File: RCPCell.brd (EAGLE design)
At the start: 99.8 x 80 mm, 23 parts, among them IC1 SIM900, Q1 BSS84, Q2 BSS84, U1 PESDXS4UD

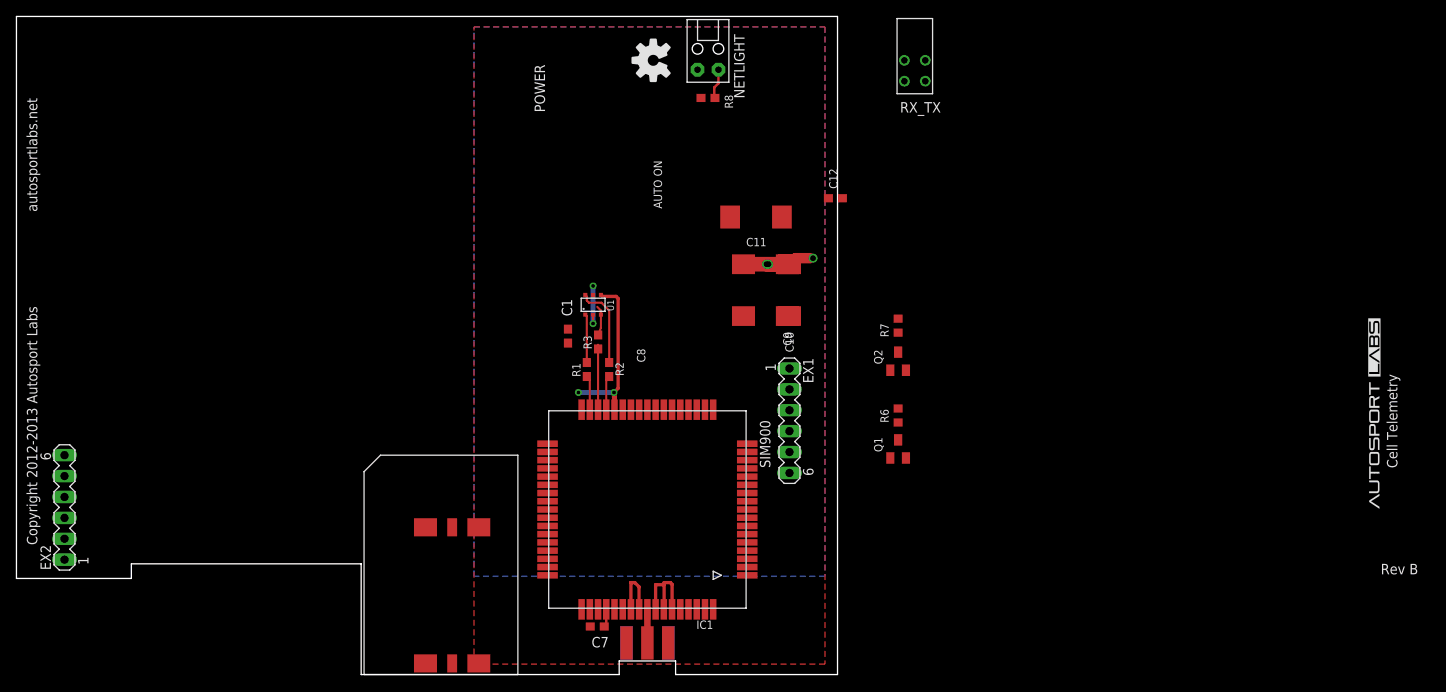
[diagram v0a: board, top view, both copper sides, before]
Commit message: WIP for MK2 version of cell module
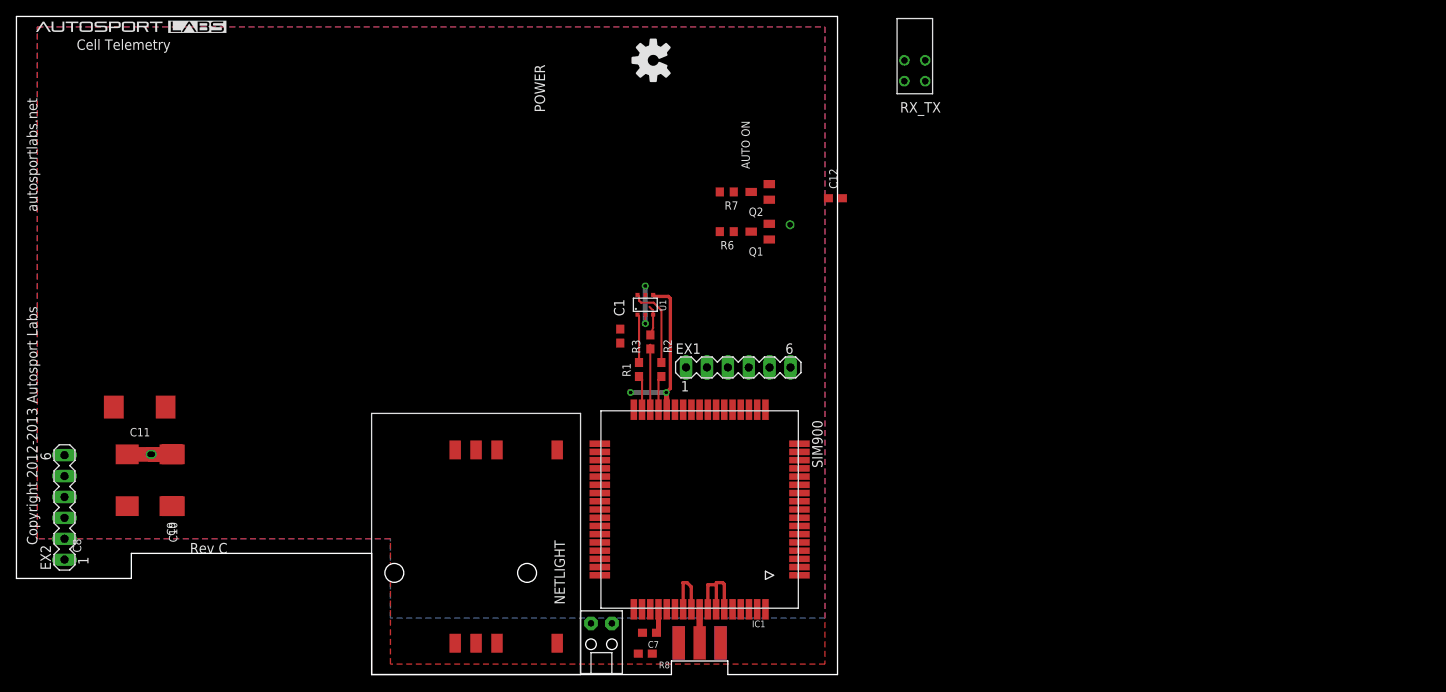
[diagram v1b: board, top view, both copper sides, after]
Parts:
- U$1: value MOLEX_0470230001 -> MOLEX_04702300012; device simcard:MOLEX_0470230001 -> simcard:MOLEX_91228-3001
- moved C10 78.4 mm to (19.1, 23.6)
- moved C9 78.4 mm to (18.8, 23.6)
- moved C11 78.4 mm to (15.0, 32.5)
- moved C8 78.4 mm to (13.5, 23.6)
- moved NETLIGHT 71.8 mm to (71.1, 4.57), turned to 0 degrees
- moved R8 68.0 mm to (76.5, 2.54)
- moved Q1 31.3 mm to (90.4, 53.8), turned to 90 degrees
- moved R6 30.6 mm to (86.4, 53.8), turned to 180 degrees
- moved Q2 26.5 mm to (90.4, 58.7), turned to 90 degrees
- moved R7 26.4 mm to (86.4, 58.7), turned to 180 degrees
- moved EX1 8.98 mm to (87.8, 37.3), turned to 0 degrees
- moved U$1 8.52 mm to (53.3, 3.81), turned to 0 degrees
- moved C7 6.40 mm to (77.0, 5.08)
- moved C1 6.35 mm to (73.4, 41.1)
- moved IC1 6.35 mm to (83.1, 20.1)
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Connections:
- removed net N$2: NETLIGHT.A, R8.1
- new net N$1: NETLIGHT.C, R8.2
- net GND: now also R8.1; no longer NETLIGHT.C
- net STATUS: now also NETLIGHT.A; no longer R8.2
- net USB_DM_HS_OUT: now also EX1.3; no longer EX1.4
- net USB_DP_HS_OUT: now also EX1.4; no longer EX1.3
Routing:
- net N$2: track 3.68 -> 0.00 mm
- net V+: track 13.6 -> 11.2 mm
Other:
- outline, holes or cut-outs redrawn
- board text added: "Rev C"
- board text removed: "Rev B"
